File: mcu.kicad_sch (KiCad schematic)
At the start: 16 parts, among them IC1 STM32C542CCT6, J8 Conn_02x05_Odd_Even, SW1 SW_Push, Y3 ECS-400-18-33-JGN-TR

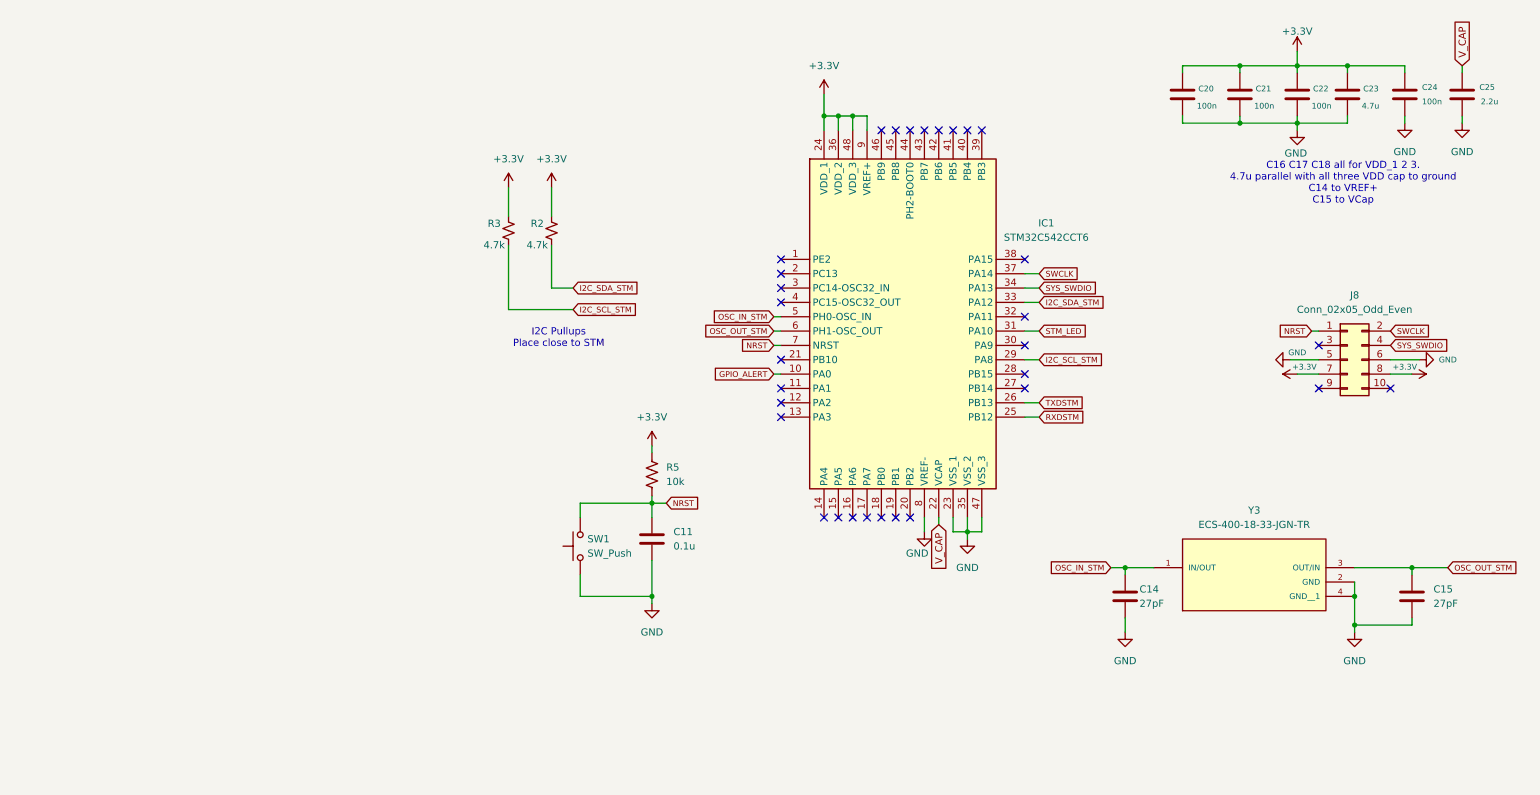
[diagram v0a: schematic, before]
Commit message: Relatively final changes
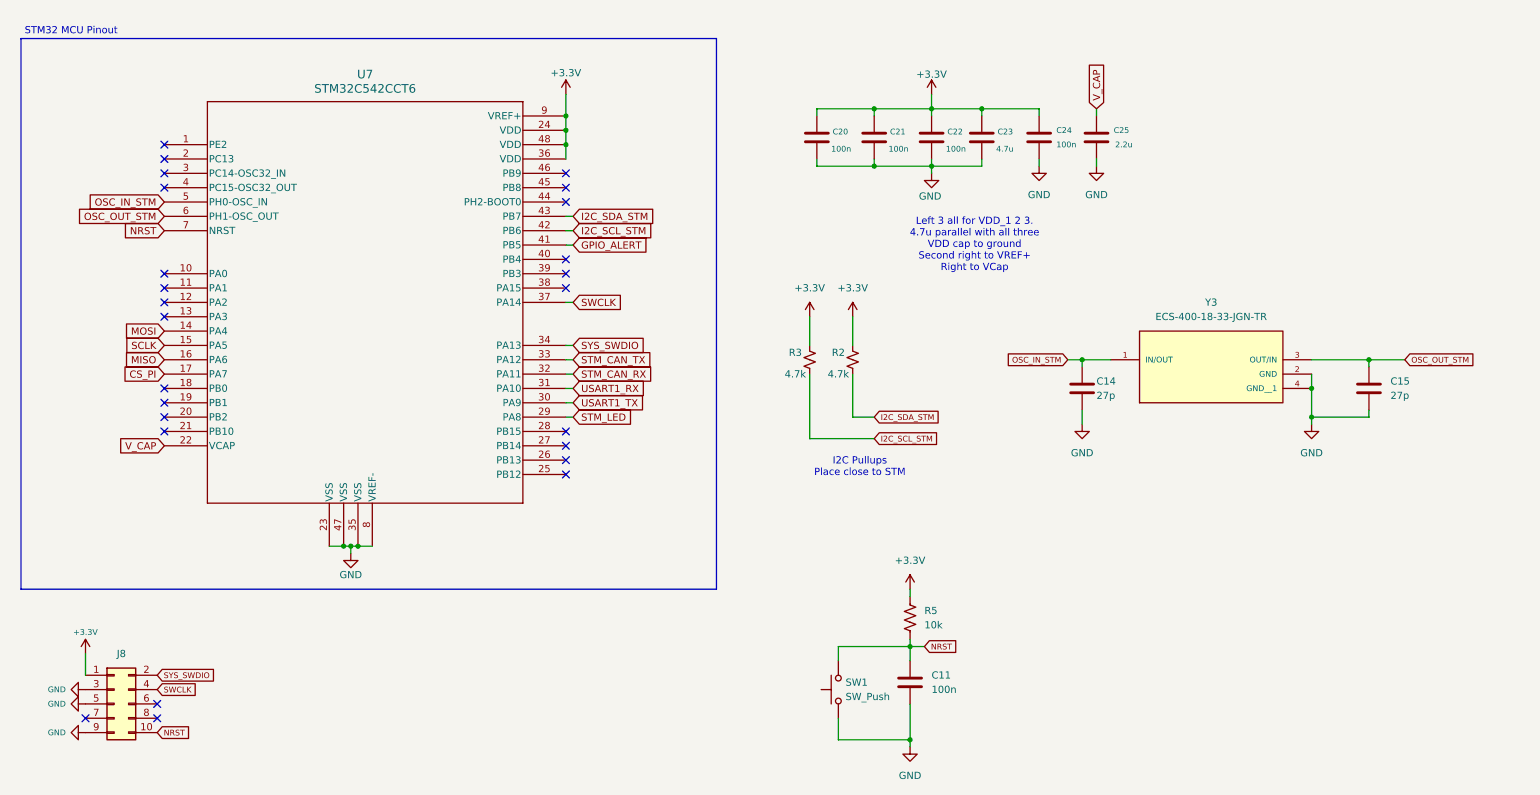
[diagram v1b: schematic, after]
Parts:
- removed IC1: STM32C542CCT6, QFP50P900X900X160-48N, symbol STM32C542CCT6:STM32C542CCT6
- added U7: STM32C542CCT6, LQFP48-7X7, symbol 2026-09-19_00-19-05:STM32C542CCT6
- C11: value 0.1u -> 100n
- C14, C15: value 27pF -> 27p
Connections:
- net +3.3V: now also J8.1 (Pin_1), U7.24 (VDD), U7.36 (VDD), U7.48 (VDD), U7.9 (VREF+); no longer J8.7 (Pin_7), J8.8 (Pin_8)
- net GND: now also J8.3 (Pin_3), J8.9 (Pin_9), U7.23 (VSS), U7.35 (VSS), U7.47 (VSS), U7.8 (VREF-); no longer J8.6 (Pin_6)
- net GPIO_ALERT: now also U7.41 (PB5)
- net I2C_SCL_STM: now also U7.42 (PB6)
- net I2C_SDA_STM: now also U7.43 (PB7)
- net NRST: now also J8.10 (Pin_10), U7.7 (NRST); no longer J8.1 (Pin_1)
- net OSC_IN_STM: now also U7.5 (PH0-OSC_IN)
- net OSC_OUT_STM: now also U7.6 (PH1-OSC_OUT)
- net STM_LED: now also U7.29 (PA8)
- net SWCLK: now also J8.4 (Pin_4), U7.37 (PA14); no longer J8.2 (Pin_2)
- net SYS_SWDIO: now also J8.2 (Pin_2), U7.34 (PA13); no longer J8.4 (Pin_4)
- net V_CAP: now also U7.22 (VCAP)
- new net CS_PI: U7.17 (PA7)
- new net MISO: U7.16 (PA6)
- new net MOSI: U7.14 (PA4)
- new net SCLK: U7.15 (PA5)
- new net STM_CAN_RX: U7.32 (PA11)
- new net STM_CAN_TX: U7.33 (PA12)
- new net USART1_RX: U7.31 (PA10)
- new net USART1_TX: U7.30 (PA9)
- no-connect marks 31 -> 25
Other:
- note added: "Left 3 all for VDD_1 2 3. 4.7u parallel with all three VDD cap to ground Second right to VREF+ Right to VCap"
- note added: "STM32 MCU Pinout"
- note removed: "C16 C17 C18 all for VDD_1 2 3. 4.7u parallel with all three VDD cap to ground C14 to VREF+ C15 to VCap"
- moved on the sheet: C11, C14, C15, C20, C21, C22, C23, C24, C25, J8, R2, R3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
